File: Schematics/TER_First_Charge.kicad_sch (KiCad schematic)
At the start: 53 parts, among them M1 Fan, M2 Fan, M4 Motor_Pump, SW1 SW_SP3T, U4 MotorEncoder-RM44

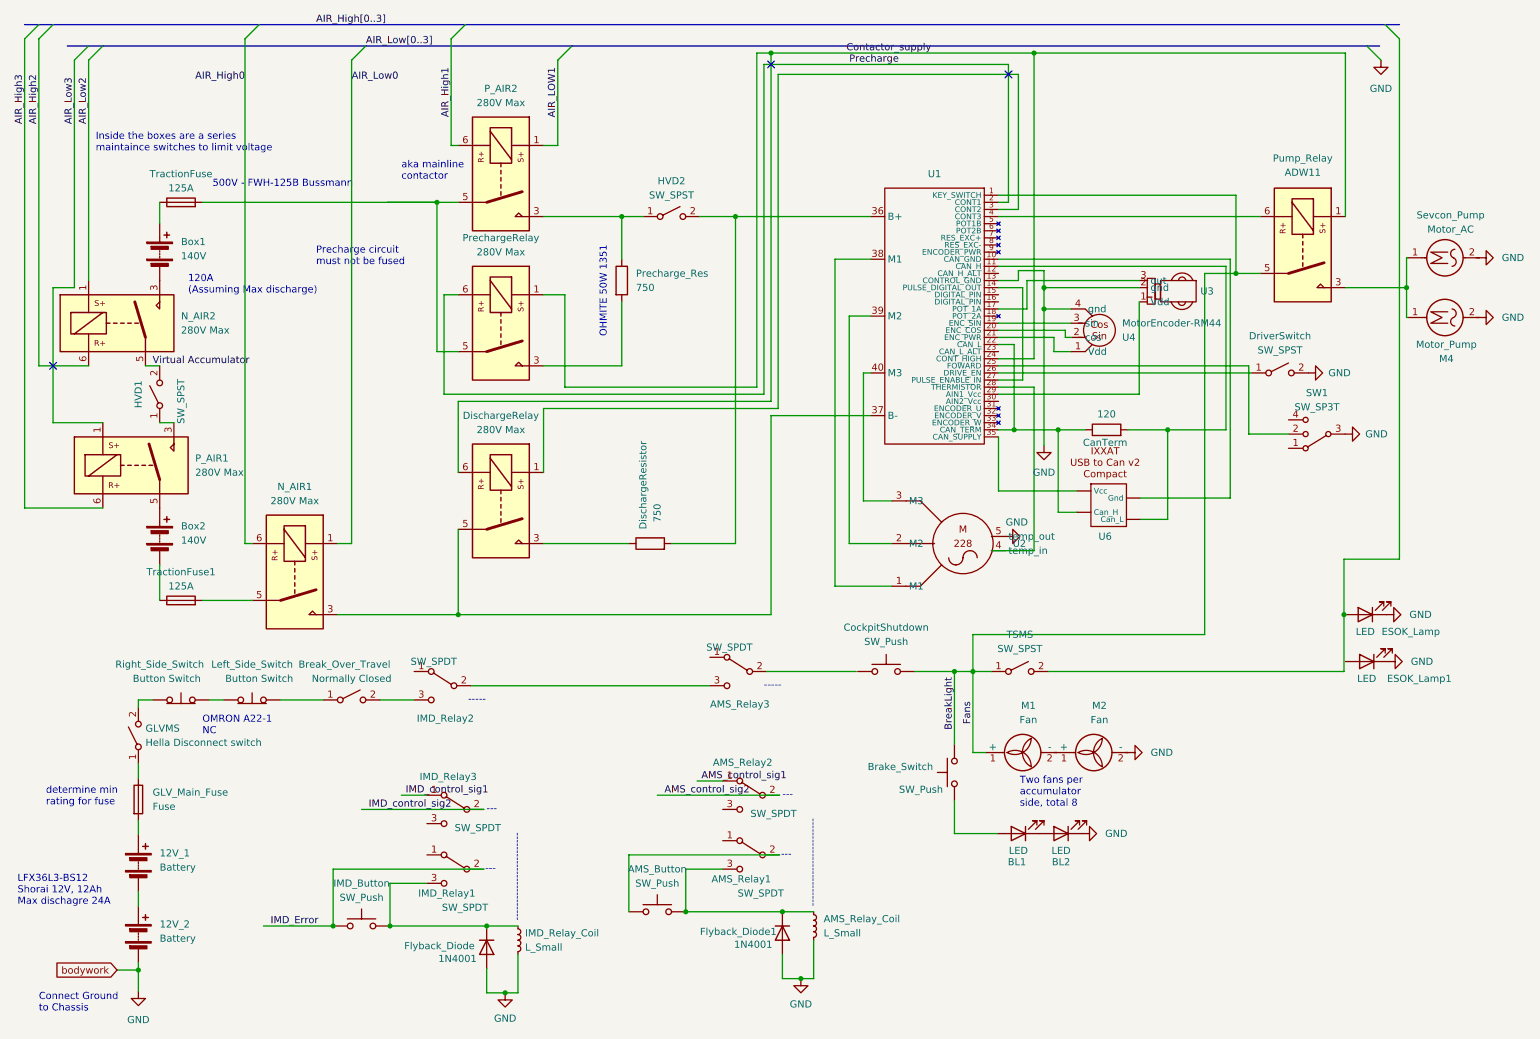
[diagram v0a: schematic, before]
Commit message: 6/7/2023, IMD Added
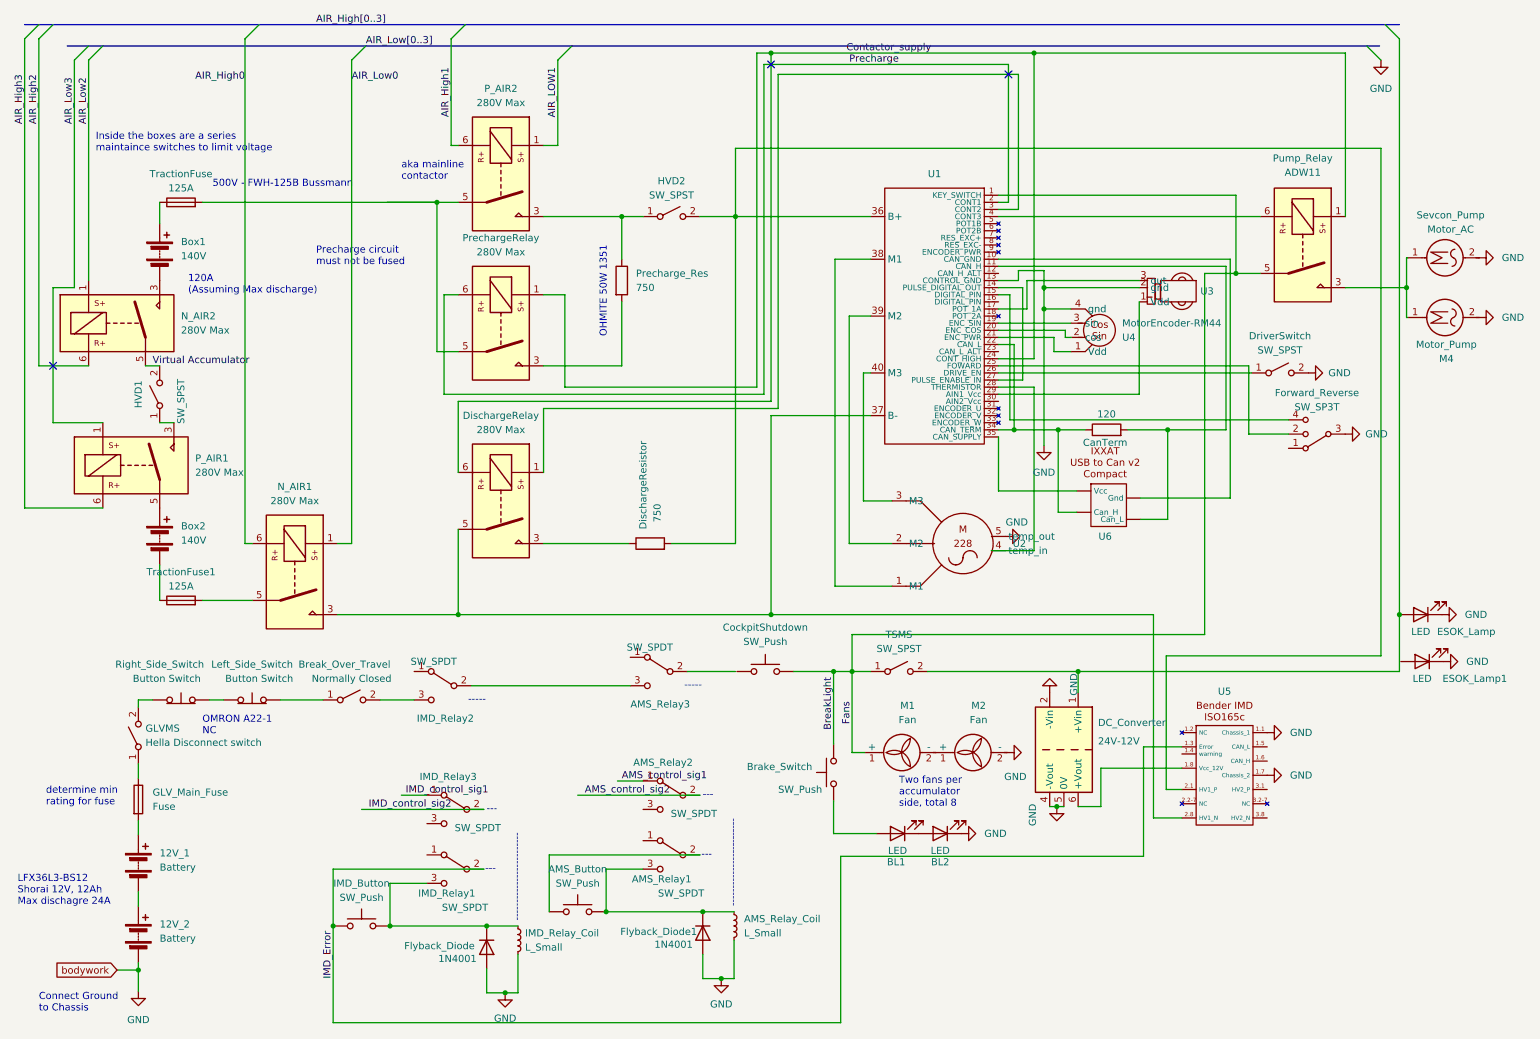
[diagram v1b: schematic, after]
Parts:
- added DC_Converter: 24V-12V, Converter_DCDC:Converter_DCDC_XP_POWER-IAxxxxS_THT, symbol Converter_DCDC:IA0503S
- added U5: ~, symbol TER:IMD
- renumbered SW1 to Forward_Reverse
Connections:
- net GND: now also DC_Converter.2 (-Vin), DC_Converter.4 (-Vout), DC_Converter.5 (0V), U5.1.1 (Chassis_1), U5.1.7 (Chassis_2)
- net IMD_Error: now also U5.1.3 (Error)
- net at Forward_Reverse.4: now also U1.15 (DIGITAL_PIN)
- net at ESOK_Lamp.2 (A), TSMS.2 (B): now also DC_Converter.1 (+Vin)
- net at DischargeRelay.5, N_AIR1.3, U1.37 (B-): now also U5.2.8 (HV1_N)
- net at DischargeResistor.2, HVD2.2 (B), U1.36 (B+): now also U5.2.1 (HV1_P)
- new net: DC_Converter.6 (+Vout), U5.1.8 (Vcc_12V)
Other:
- moved on the sheet: AMS_Button, AMS_Relay1, AMS_Relay2, AMS_Relay3, AMS_Relay_Coil, BL1, BL2, Brake_Switch, CockpitShutdown, ESOK_Lamp, ESOK_Lamp1, Flyback_Diode1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
